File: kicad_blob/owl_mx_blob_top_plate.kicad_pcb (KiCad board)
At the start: 2 copper layers, 152.1 x 123.2 mm, 23 parts

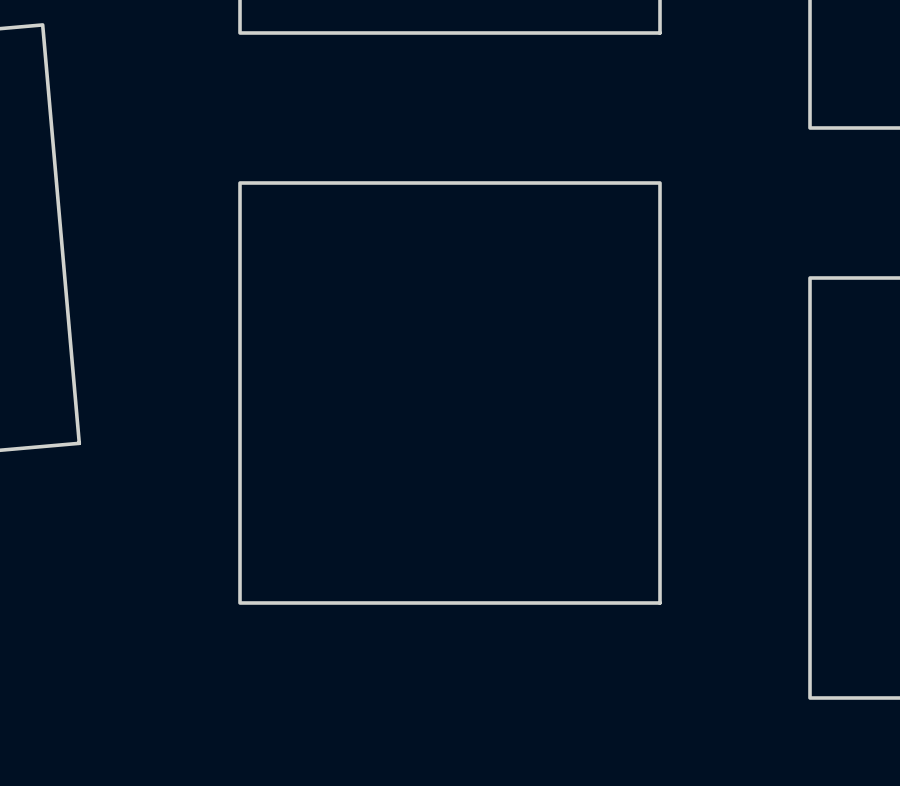
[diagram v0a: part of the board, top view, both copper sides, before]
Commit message: in progress
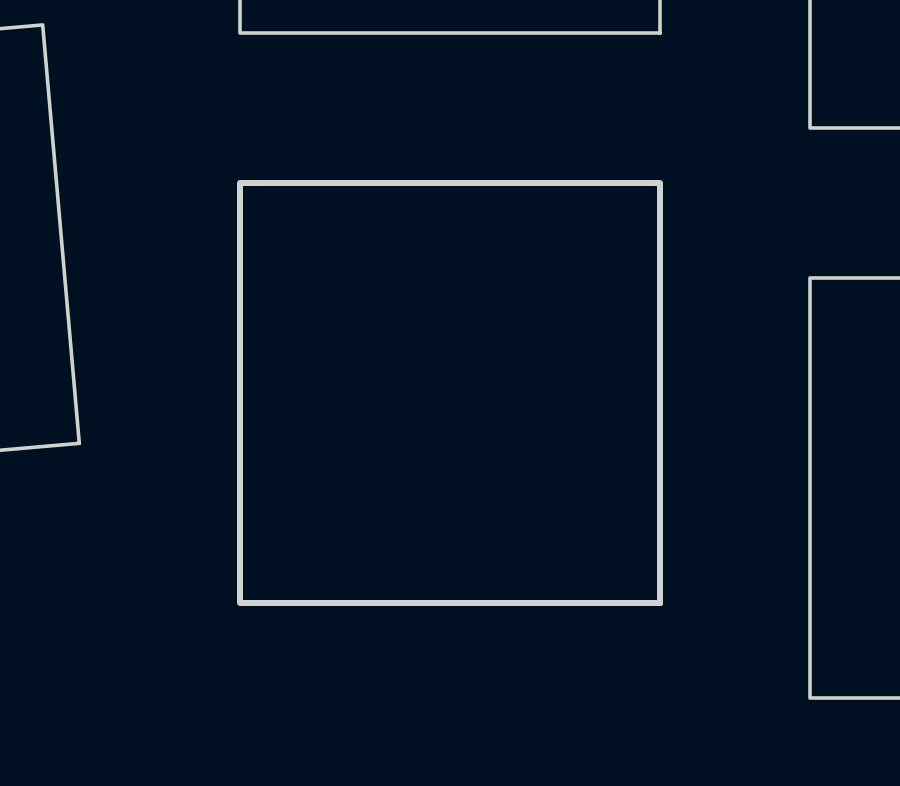
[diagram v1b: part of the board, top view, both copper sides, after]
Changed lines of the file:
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@@
     (fp_line (start 7 -7) (end 7 -6) (layer "Dwgs.User") (width 0.15))
     (fp_line (start -7 7) (end -6 7) (layer "Dwgs.User") (width 0.15))
-    (fp_rect (start -7 -7) (end 7 7) (layer "Edge.Cuts") (width 0.12) (fill none))
+    (fp_rect (start -7 -7) (end 7 7) (layer "Edge.Cuts") (width 0.2) (fill none))
   )
   (footprint "SMDPad" (layer "F.Cu")
